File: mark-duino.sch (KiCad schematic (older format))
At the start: 57 parts, among them IC1 ATmega328P, J1 Conn_FTDI, J2 IC1_Analog, J3 IC1_SPI, J4 IC1_Digital, J5 12VDC_IN, J6 IC1_I2C, J7 Conn_12V, J8 MCP_Analog, J9 Conn_5V, SW1 SW_SPDT, U1 MCP3008, Y1 16MHz

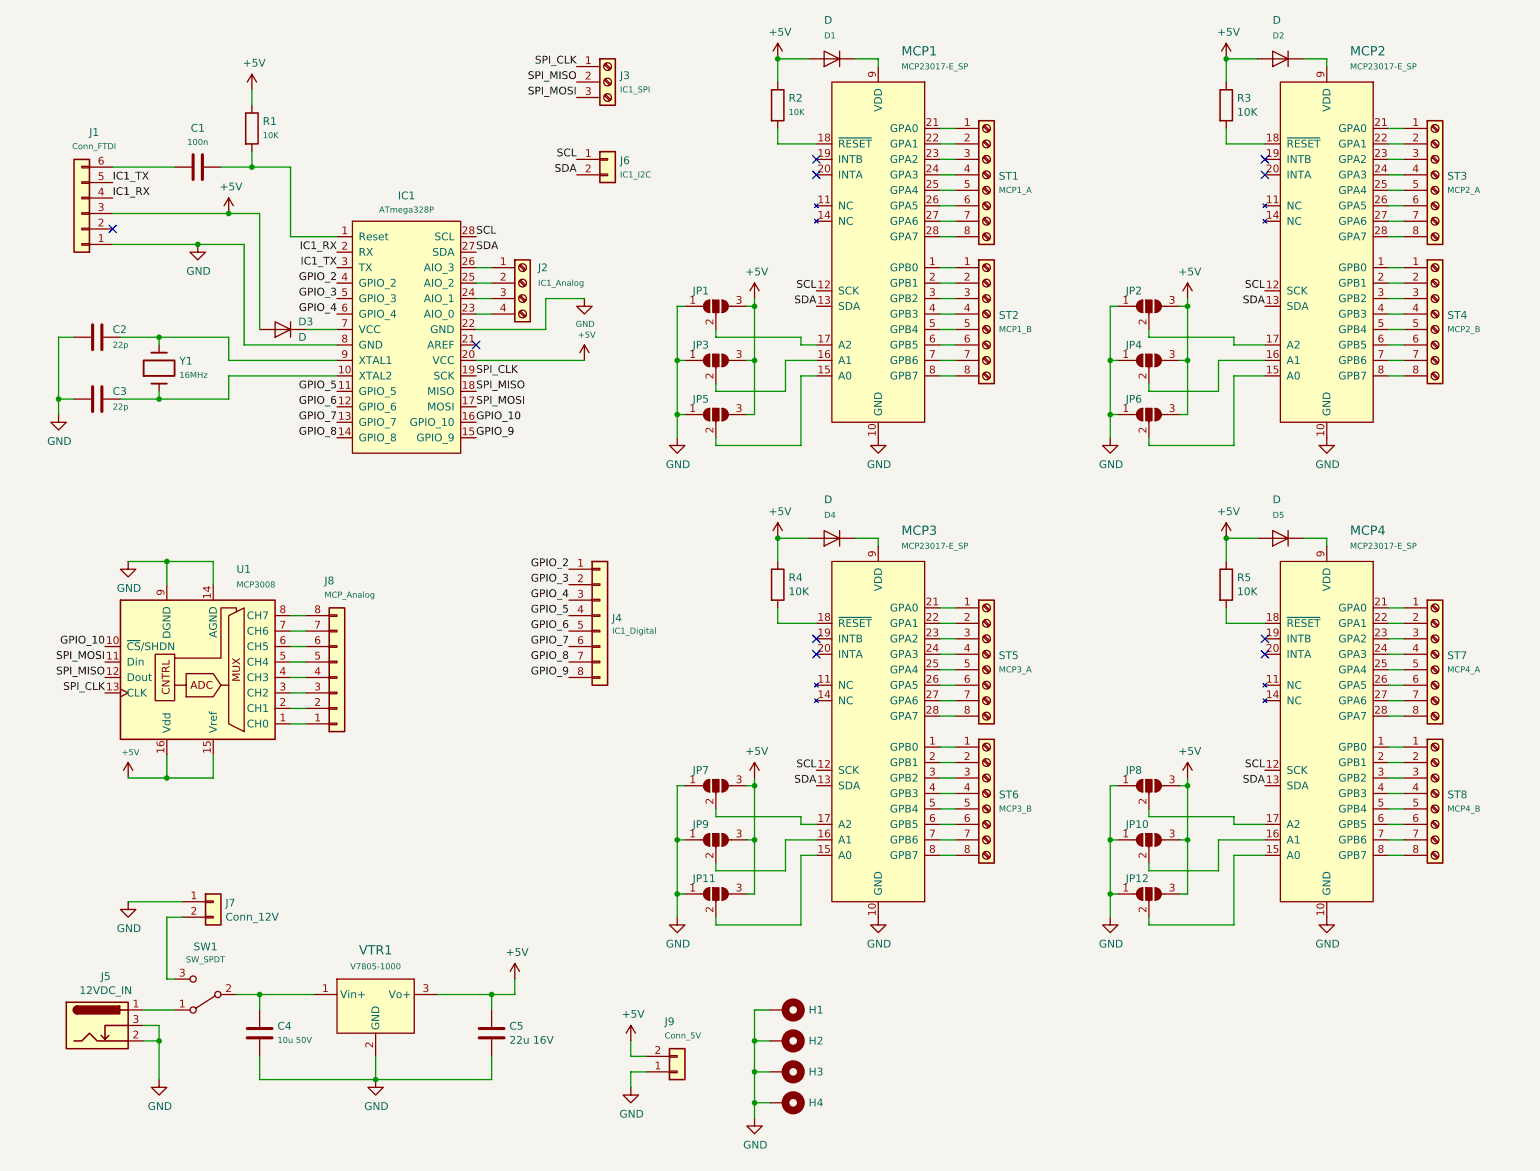
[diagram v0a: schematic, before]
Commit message: Cleaned up and updated documentation
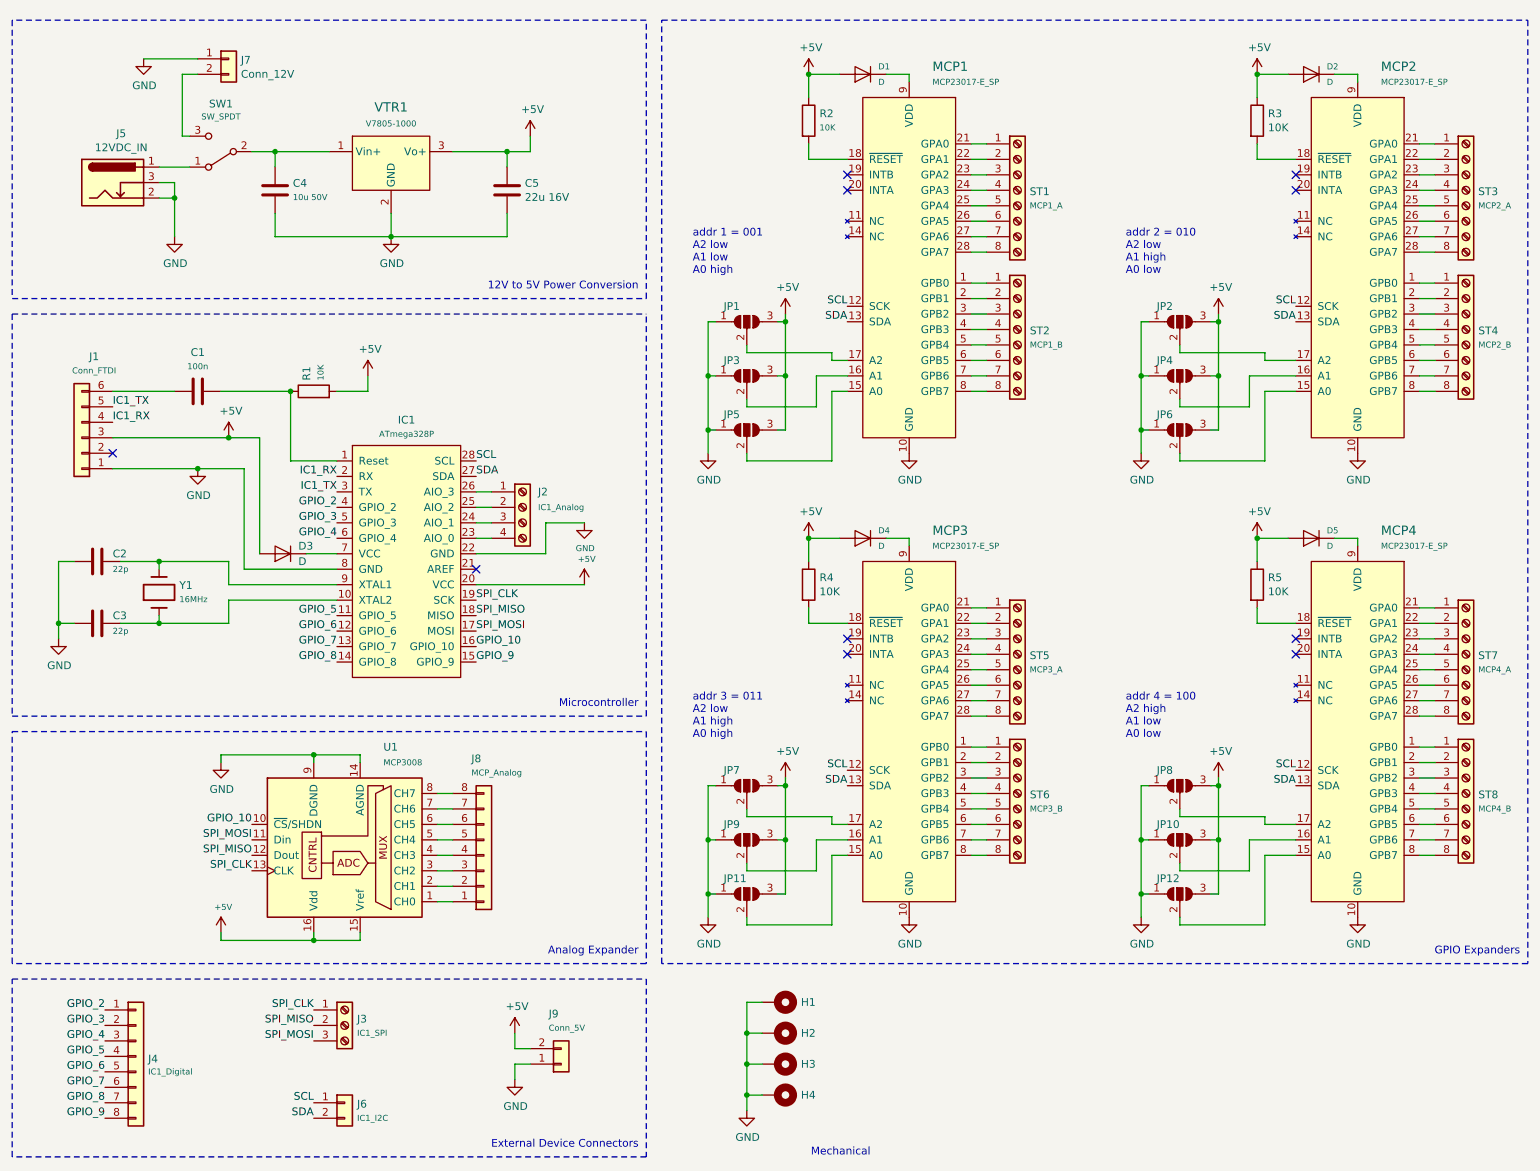
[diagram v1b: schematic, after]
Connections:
- net +5V: now also R1.2; no longer R1.1
- net at C1.1, IC1.1 (Reset): now also R1.1; no longer R1.2
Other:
- note added: "12V to 5V Power Conversion"
- note added: "Analog Expander"
- note added: "External Device Connectors"
- note added: "GPIO Expanders"
- note added: "Mechanical"
- note added: "Microcontroller"
- note added: "addr 1 = 001\nA2 low\nA1 low\nA0 high"
- note added: "addr 2 = 010\nA2 low\nA1 high\nA0 low"
- note added: "addr 3 = 011\nA2 low\nA1 high\nA0 high"
- note added: "addr 4 = 100\nA2 high\nA1 low\nA0 low"
- moved on the sheet: C1, C2, C3, C4, C5, D1, D2, D3, D4, D5, H1, H2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
